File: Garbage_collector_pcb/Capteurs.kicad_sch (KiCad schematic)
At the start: 8 parts, among them J10 TOF2, J11 Lidar, J12 TOF3, J13 NeoPixel, J8 TOF1, J9 TOF+Couleur

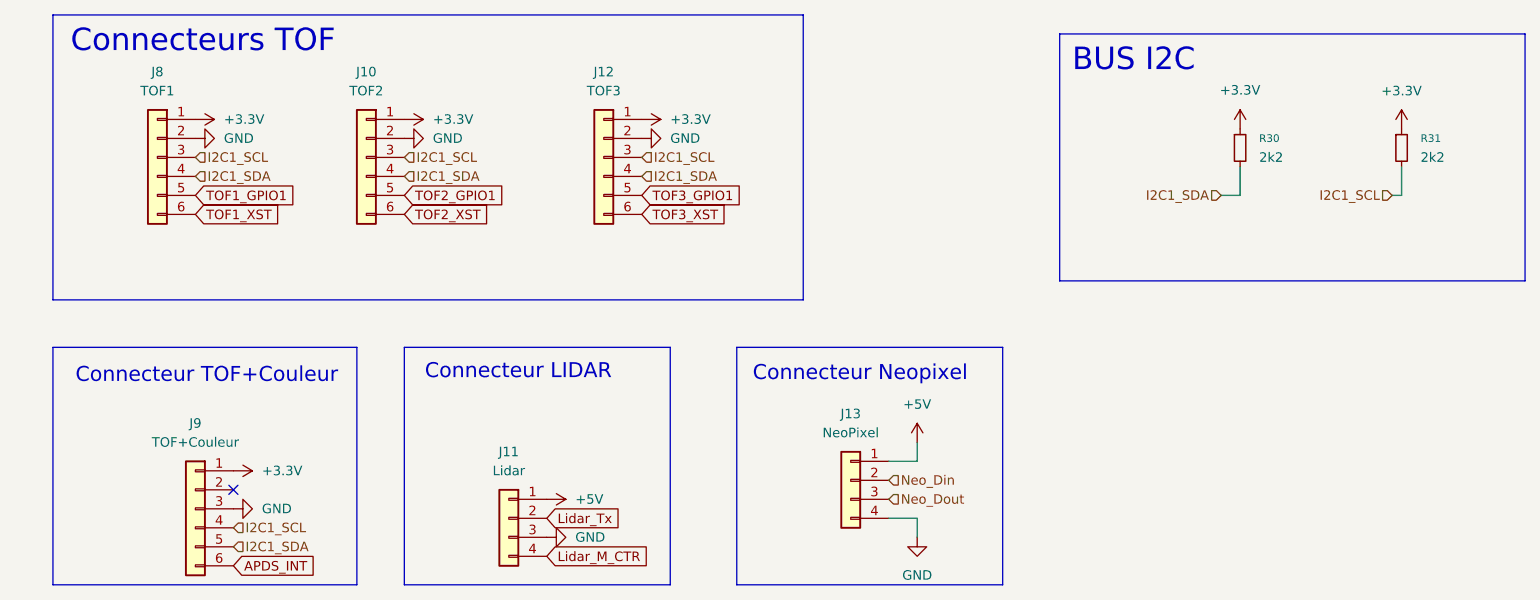
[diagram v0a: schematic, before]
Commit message: ajout du ioc et schema validé
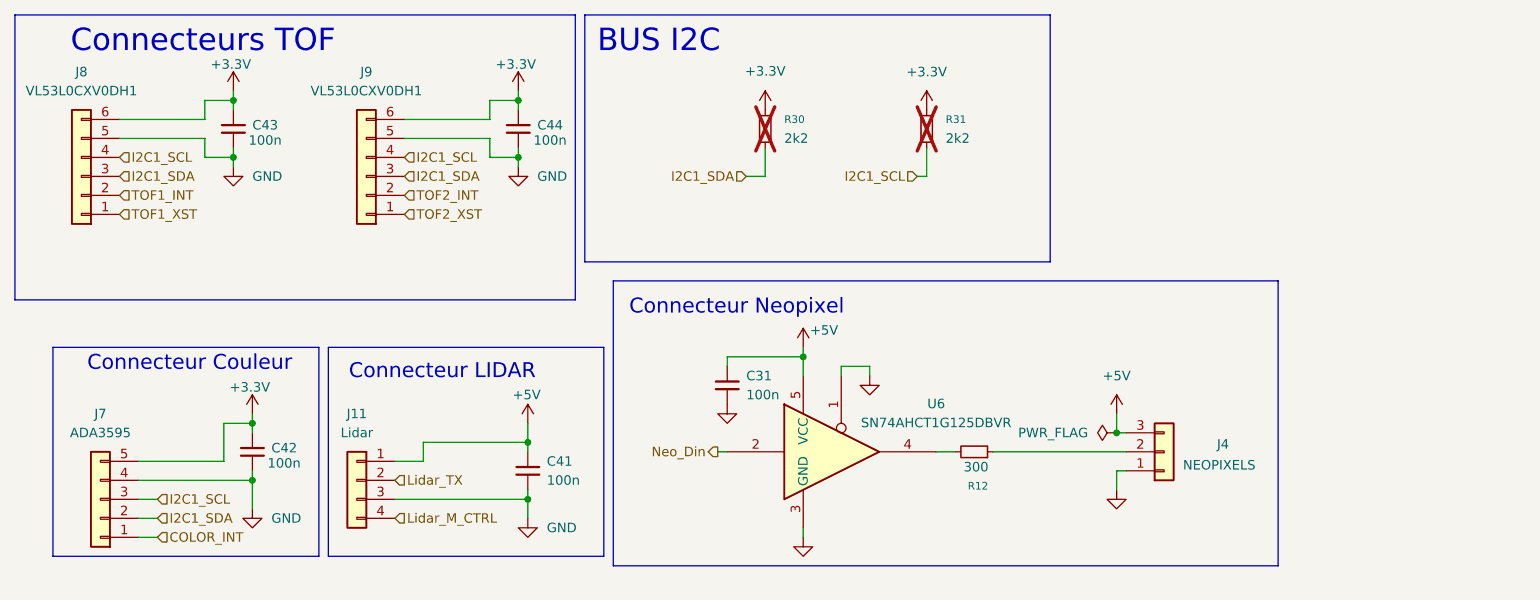
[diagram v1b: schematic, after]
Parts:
- removed J10: TOF2, symbol Kicad:Conn_01x06
- removed J12: TOF3, symbol Kicad:Conn_01x06
- removed J13: NeoPixel, symbol Kicad:Conn_01x04
- removed J8: TOF1, symbol Kicad:Conn_01x06
- removed J9: TOF+Couleur, symbol Kicad:Conn_01x06
- added C31, C41, C42, C43, C44: 100n, Capacitor_SMD:C_0402_1005Metric, symbol Device:C_Small
- added J4: NEOPIXELS, Connector_JST:JST_GH_SM03B-GHS-TB_1x03-1MP_P1.25mm_Horizontal, symbol Connector_Generic:Conn_01x03
- added J7: ADA3595, Connector_JST:JST_GH_SM05B-GHS-TB_1x05-1MP_P1.25mm_Horizontal, symbol Connector_Generic:Conn_01x05
- added J8, J9: VL53L0CXV0DH1, Connector_JST:JST_GH_SM06B-GHS-TB_1x06-1MP_P1.25mm_Horizontal, symbol Connector_Generic:Conn_01x06
- added R12: 300, Resistor_SMD:R_0603_1608Metric, symbol Device:R_Small
- added U6: SN74AHCT1G125DBVR, Package_TO_SOT_SMD:SOT-23-5, symbol 74xGxx:74AHCT1G125
- J11: footprint (none) -> Connector_JST:JST_GH_BM04B-GHS-TBT_1x04-1MP_P1.25mm_Vertical
- R30, R31: JLCPCB Part # (none) -> C25879; now not fitted
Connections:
- net +3.3V: now also C42.1, C43.1, C44.1, J7.5 (Pin_5), J8.6 (Pin_6), J9.6 (Pin_6)
- net +5V: now also C31.1, C41.1, J4.3 (Pin_3), U6.5 (VCC)
- net GND: now also C31.2, C41.2, C42.2, C43.2, C44.2, J4.1 (Pin_1), J7.4 (Pin_4), J8.5 (Pin_5), J9.5 (Pin_5), U6.1, U6.3 (GND)
- net I2C1_SCL: now also J7.3 (Pin_3), J8.4 (Pin_4), J9.4 (Pin_4)
- net I2C1_SDA: now also J7.2 (Pin_2), J8.3 (Pin_3), J9.3 (Pin_3)
- net Neo_Din: now also U6.2
- net TOF1_XST: now also J8.1 (Pin_1)
- net TOF2_XST: now also J9.1 (Pin_1)
- net Lidar_M_CTR renamed Lidar_M_CTRL
- net Lidar_Tx renamed Lidar_TX
- new net: J4.2 (Pin_2), R12.1
- new net: R12.2, U6.4
- new net COLOR_INT: J7.1 (Pin_1)
- new net TOF1_INT: J8.2 (Pin_2)
- new net TOF2_INT: J9.2 (Pin_2)
- no-connect marks 1 -> 0
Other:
- note added: "Connecteur Couleur"
- note removed: "Connecteur TOF+Couleur"
- moved on the sheet: J11
